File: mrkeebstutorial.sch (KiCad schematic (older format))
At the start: 153 parts, among them J1 USB_B_Mini, SW1 tilde/esc, SW10 9, SW11 0, SW12 _, SW13 =/+, SW14 Backspace_200, SW15 M1, SW16 Tab_150, SW17 Q, SW18 W, SW19 E, SW2 1, SW20 R, SW21 T, SW22 Y, SW23 U, SW24 I, SW25 O, SW26 P, SW27 {, SW28 }, SW29 \\, SW3 2, SW30 M2, SW31 Caps, SW32 A, SW33 S, SW34 D, SW35 F, SW36 G, SW37 H, SW38 J, SW39 K, SW4 3, SW40 L, SW41 :, SW42 \", SW43 Enter_2.25, SW44 M3, SW45 LShift_225, SW46 z, SW47 x, SW48 c, SW49 v, SW5 4, SW50 b, SW51 n, SW52 m, SW53 <, SW54 >, SW55 ?, SW56 R-shift_175, SW57 UP, SW58 M4, SW59 LCTRL, SW6 5, SW60 Win, SW61 Alt, SW62 Space, SW63 Alt, SW64 Win, SW65 Menu, SW66 LEFT, SW67 DOWN, SW68 RIGHT, SW7 6, SW8 7, SW9 8, U1 ATmega32U4-AU, Y1 16MHz

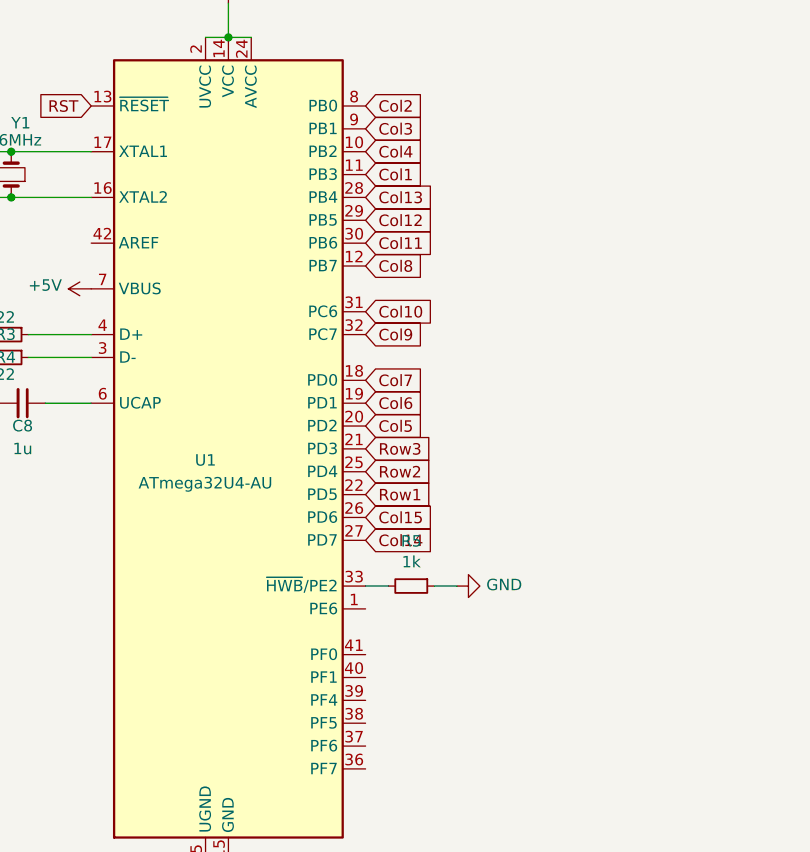
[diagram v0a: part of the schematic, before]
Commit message: rearranged
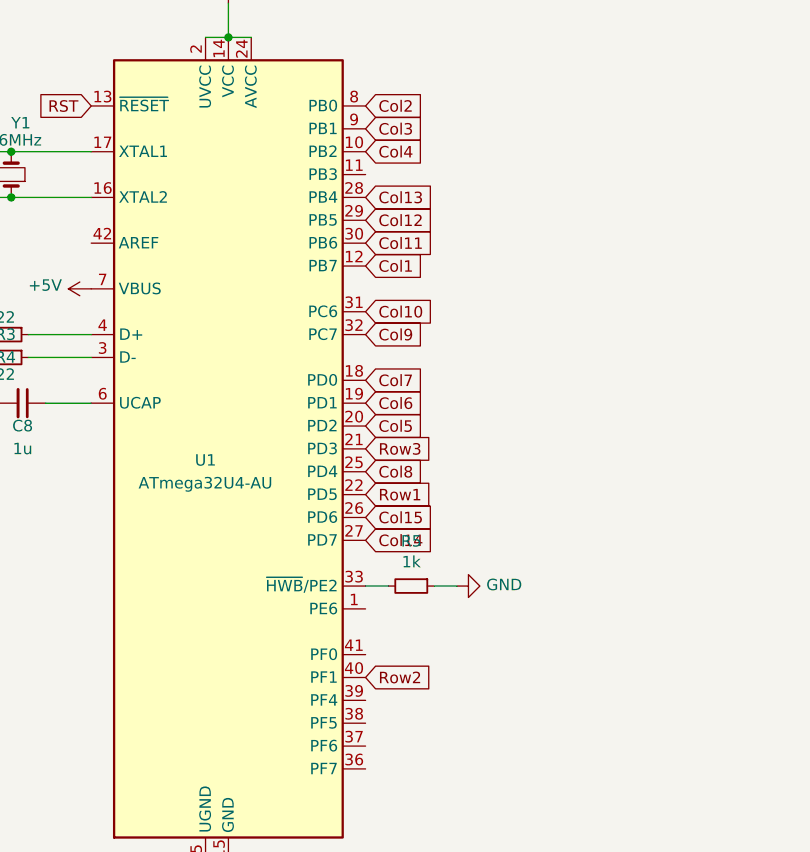
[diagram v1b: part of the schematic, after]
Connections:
- net Col1: now also U1.12 (PB7); no longer U1.11 (PB3)
- net Col8: now also U1.25 (PD4); no longer U1.12 (PB7)
- net Row2: now also U1.40 (PF1); no longer U1.25 (PD4)
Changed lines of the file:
@@
 Text GLabel -1000 2900 2    50   Input ~ 0
 Row3
-Text GLabel -1000 3000 2    50   Input ~ 0
+Text GLabel -1000 3900 2    50   Input ~ 0
 Row2
 Text GLabel -1000 3100 2    50   Input ~ 0
@@
 Text GLabel -1000 2300 2    50   Input ~ 0
 Col10
-Text GLabel -1000 2100 2    50   Input ~ 0
-Col8
 Text GLabel -1000 2600 2    50   Input ~ 0
 Col7
@@
 Wire Wire Line
 	14925 4325 15850 4325
-Text GLabel -1000 1700 2    50   Input ~ 0
+Text GLabel -1000 2100 2    50   Input ~ 0
 Col1
 Text GLabel -1000 1400 2    50   Input ~ 0
@@
 	1    0    0    -1
 $EndComp
+Text GLabel -1000 3000 2    50   Input ~ 0
+Col8
 Text GLabel -1000 2000 2    50   Input ~ 0
 Col11
